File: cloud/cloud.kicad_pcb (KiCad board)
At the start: 2 copper layers, 70 x 50 mm, 33 parts, among them J3 USB_C_Receptacle_USB2.0_16P, SW5 SW_Push, SW6 SW_Push, U1 ESP32-S3-WROOM-1, U2 AZ1117CH2-3.3

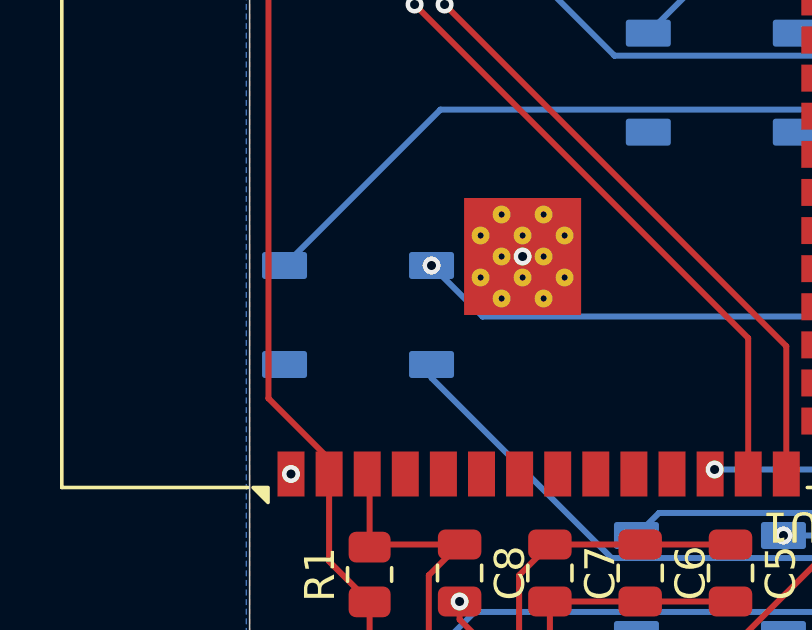
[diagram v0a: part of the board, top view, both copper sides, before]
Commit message: update pcb
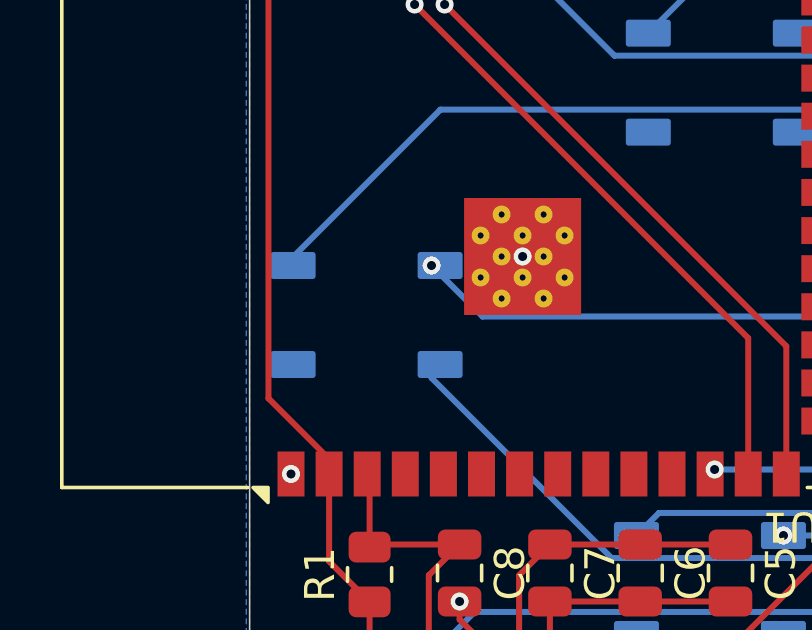
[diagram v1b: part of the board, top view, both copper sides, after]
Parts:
- moved D16 0.29 mm to (123.9, 64.3)
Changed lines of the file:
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@@
 	(footprint "LED_SMD:LED_WS2812B_PLCC4_5.0x5.0mm_P3.2mm"
 		(layer "B.Cu")
-		(at 123.615 64.35 180)
+		(at 123.9 64.35 180)
 		(descr "5.0mm x 5.0mm Addressable RGB LED NeoPixel, https://cdn-shop.adafruit.com/datasheets/WS2812B.pdf")
 		(tags "LED RGB NeoPixel PLCC-4 5050")
